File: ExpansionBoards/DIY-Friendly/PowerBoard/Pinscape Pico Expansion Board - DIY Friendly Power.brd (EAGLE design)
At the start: 138 x 100 mm, 79 parts, among them IC1 UCC27524P, IC10 ULN2803A, IC11 ULN2803A, IC12 ULN2803A, IC13 DS1307+, IC2 UCC27524P, IC3 UCC27524P, IC4 UCC27524P, IC5 UCC27524P, IC6 UCC27524P, IC7 UCC27524P, IC8 UCC27524P, IC9 ULN2803A, J1 640445-6, J15 SSQ-108-02-T-S-RA, J2 640445-9, J3 640445-9, J4 1-640456-0, J5 1-640456-0, J6 1-640456-0, J7 1-640456-0, Q1 FDPF085N10A, Q10 FDPF085N10A, Q11 FDPF085N10A, Q12 FDPF085N10A, Q13 FDPF085N10A, Q14 FDPF085N10A, Q15 FDPF085N10A, Q16 FDPF085N10A, Q2 FDPF085N10A, Q3 FDPF085N10A, Q4 FDPF085N10A, Q5 FDPF085N10A, Q6 FDPF085N10A, Q7 FDPF085N10A, Q8 FDPF085N10A, Q9 FDPF085N10A, Y1 ECS-.327-12.5-13X-C

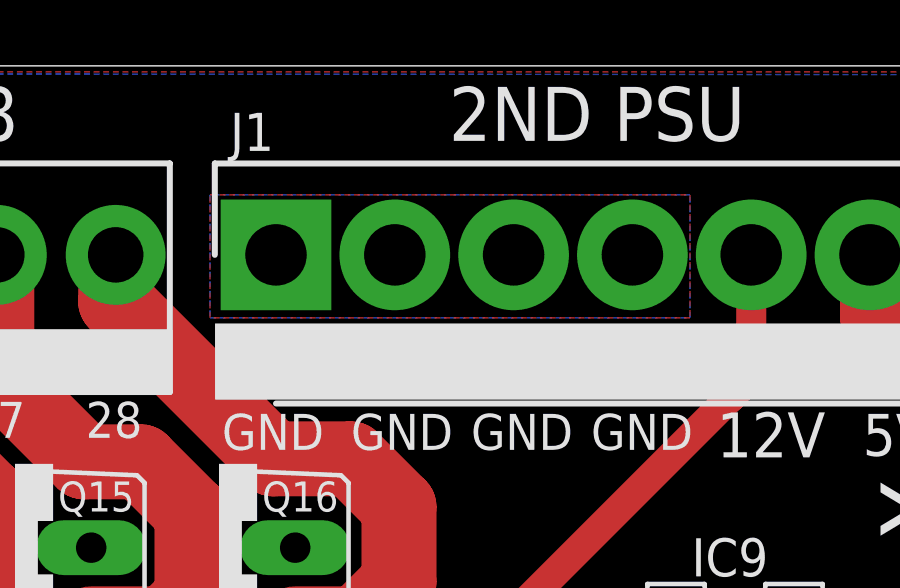
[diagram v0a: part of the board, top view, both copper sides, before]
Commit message: add logo image
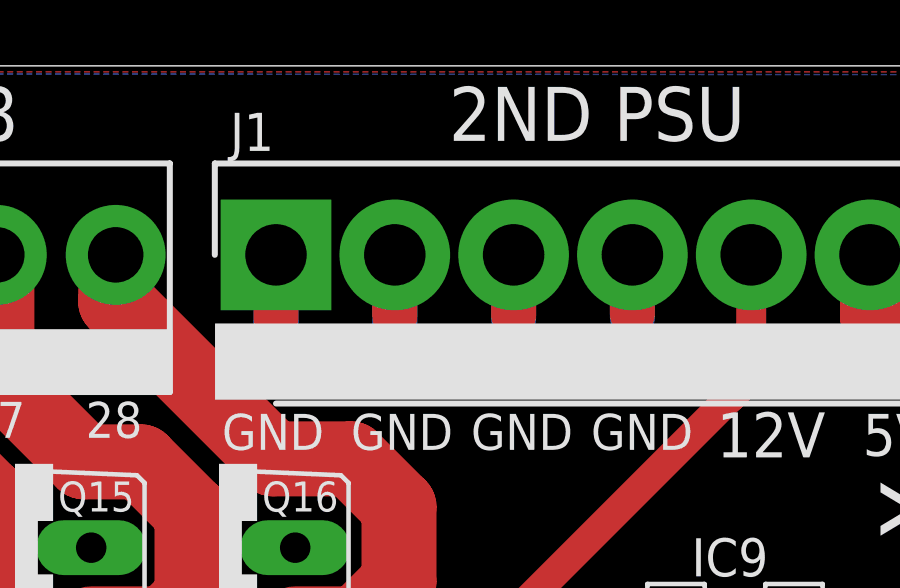
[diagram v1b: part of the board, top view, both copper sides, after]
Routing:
- net GND: track 0.00 -> 17.1 mm
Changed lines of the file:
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@@
 <contactref element="J1" pad="3"/>
 <contactref element="J1" pad="4"/>
-<polygon width="0.3" layer="1" thermals="no">
-<vertex x="103.6" y="95.7"/>
-<vertex x="119.6" y="95.7"/>
-<vertex x="119.6" y="91.6"/>
-<vertex x="103.6" y="91.6"/>
-</polygon>
-<polygon width="0.3" layer="16" thermals="no">
-<vertex x="103.6" y="91.6"/>
-<vertex x="119.6" y="91.6"/>
-<vertex x="119.6" y="95.7"/>
-<vertex x="103.6" y="95.7"/>
-</polygon>
 <polygon width="0.3" layer="16" thermals="no">
 <vertex x="12" y="23.5"/>
@@
 <vertex x="12" y="23.6"/>
 </polygon>
+<wire x1="105.8" y1="93.7" x2="105.8" y2="91.6" width="1.5" layer="1"/>
+<wire x1="109.76" y1="93.7" x2="109.76" y2="91.64" width="1.5" layer="1"/>
+<wire x1="113.72" y1="93.7" x2="113.72" y2="91.68" width="1.5" layer="1"/>
+<wire x1="117.68" y1="93.7" x2="117.68" y2="91.72" width="1.5" layer="1"/>
+<wire x1="105.8" y1="93.7" x2="105.8" y2="91.4" width="1.5" layer="16"/>
+<wire x1="109.76" y1="93.7" x2="109.76" y2="91.24" width="1.5" layer="16"/>
+<wire x1="113.72" y1="93.7" x2="113.72" y2="91.58" width="1.5" layer="16"/>
+<wire x1="117.68" y1="93.7" x2="117.68" y2="91.62" width="1.5" layer="16"/>
 </signal>
 <signal name="SDA">

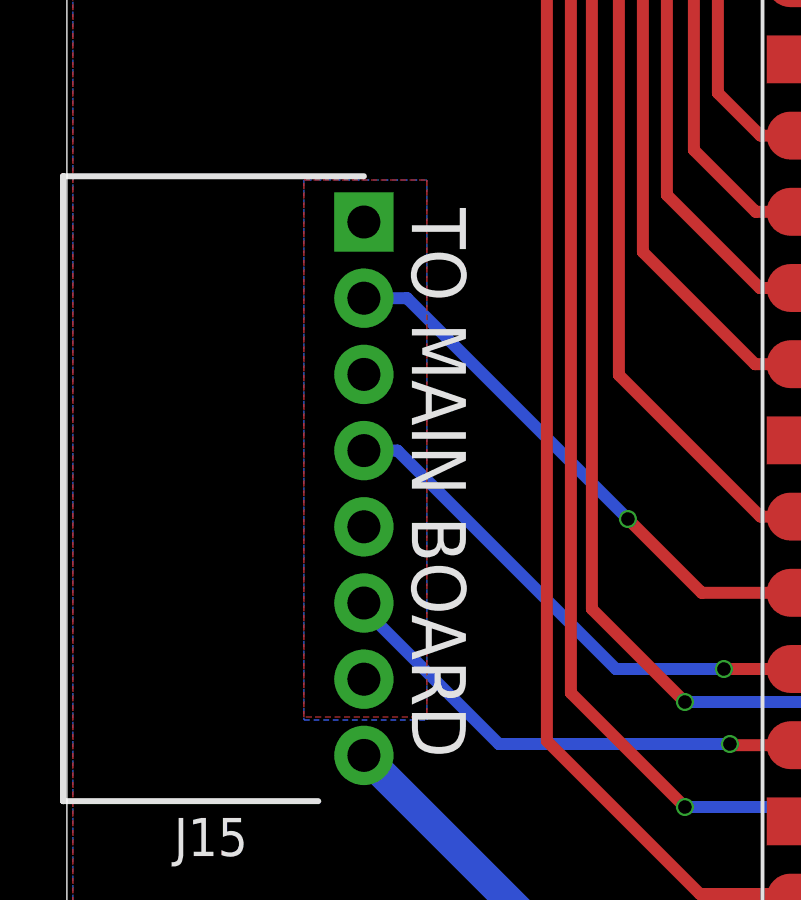
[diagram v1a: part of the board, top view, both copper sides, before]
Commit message: minor board updates
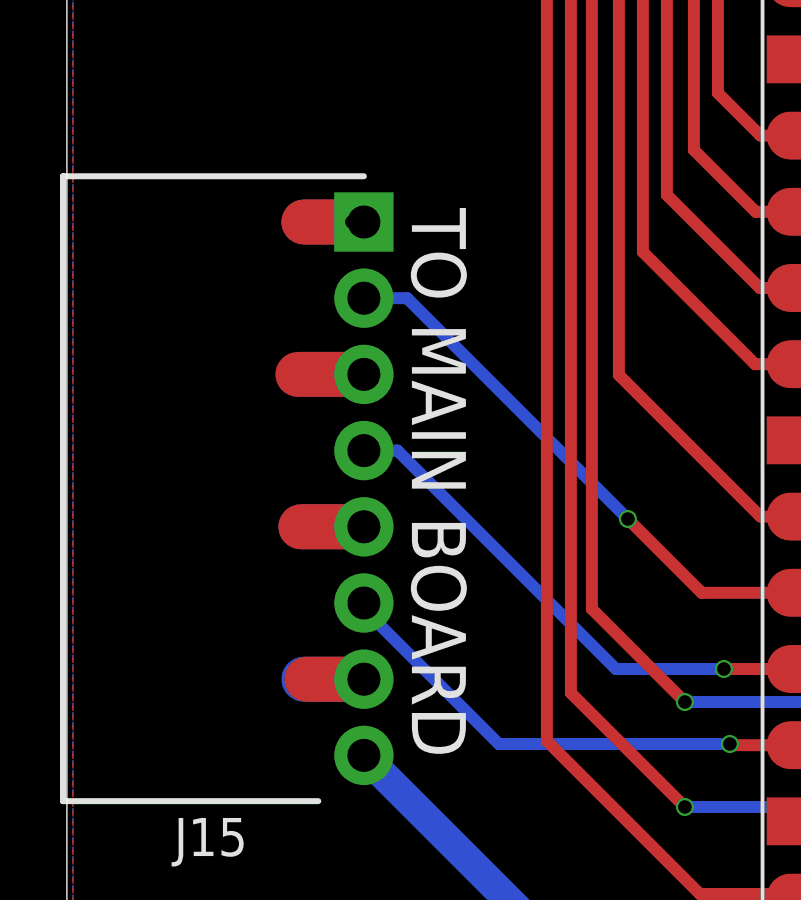
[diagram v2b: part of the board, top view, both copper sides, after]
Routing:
- net GND: track 17.1 -> 33.1 mm, vias 16 -> 17
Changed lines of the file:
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@@
 <contactref element="J1" pad="3"/>
 <contactref element="J1" pad="4"/>
-<polygon width="0.3" layer="16" thermals="no">
-<vertex x="12" y="23.5"/>
-<vertex x="12" y="41.5"/>
-<vertex x="7.9" y="41.5"/>
-<vertex x="7.9" y="23.5"/>
-</polygon>
-<polygon width="0.3" layer="1" thermals="no">
-<vertex x="7.9" y="23.6"/>
-<vertex x="7.9" y="41.5"/>
-<vertex x="12" y="41.5"/>
-<vertex x="12" y="23.6"/>
-</polygon>
 <wire x1="105.8" y1="93.7" x2="105.8" y2="91.6" width="1.5" layer="1"/>
 <wire x1="109.76" y1="93.7" x2="109.76" y2="91.64" width="1.5" layer="1"/>
@@
 <wire x1="113.72" y1="93.7" x2="113.72" y2="91.58" width="1.5" layer="16"/>
 <wire x1="117.68" y1="93.7" x2="117.68" y2="91.62" width="1.5" layer="16"/>
+<wire x1="9.9" y1="35.02" x2="7.8" y2="35.02" width="1.5" layer="16"/>
+<wire x1="9.9" y1="29.94" x2="7.8" y2="29.94" width="1.5" layer="16"/>
+<wire x1="9.9" y1="24.86" x2="7.9" y2="24.86" width="1.5" layer="16"/>
+<wire x1="9.9" y1="24.86" x2="8" y2="24.86" width="1.5" layer="1"/>
+<wire x1="9.9" y1="29.94" x2="7.8" y2="29.94" width="1.5" layer="1"/>
+<wire x1="9.9" y1="35.02" x2="7.7" y2="35.02" width="1.5" layer="1"/>
+<wire x1="9.9" y1="40.1" x2="9.5" y2="40.1" width="1.5" layer="1"/>
+<wire x1="9.5" y1="40.1" x2="7.9" y2="40.1" width="1.5" layer="1"/>
+<via x="9.5" y="40.1" extent="1-16" drill="0.45"/>
+<wire x1="9.5" y1="40.1" x2="7.9" y2="40.1" width="1.5" layer="16"/>
 </signal>
 <signal name="SDA">
